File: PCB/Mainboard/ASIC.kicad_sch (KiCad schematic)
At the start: 0 parts

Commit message: Add files via upload
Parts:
- added U21: Bowman, symbol PC110:Bowman
- added U35: Pluto, symbol PC110:Pluto

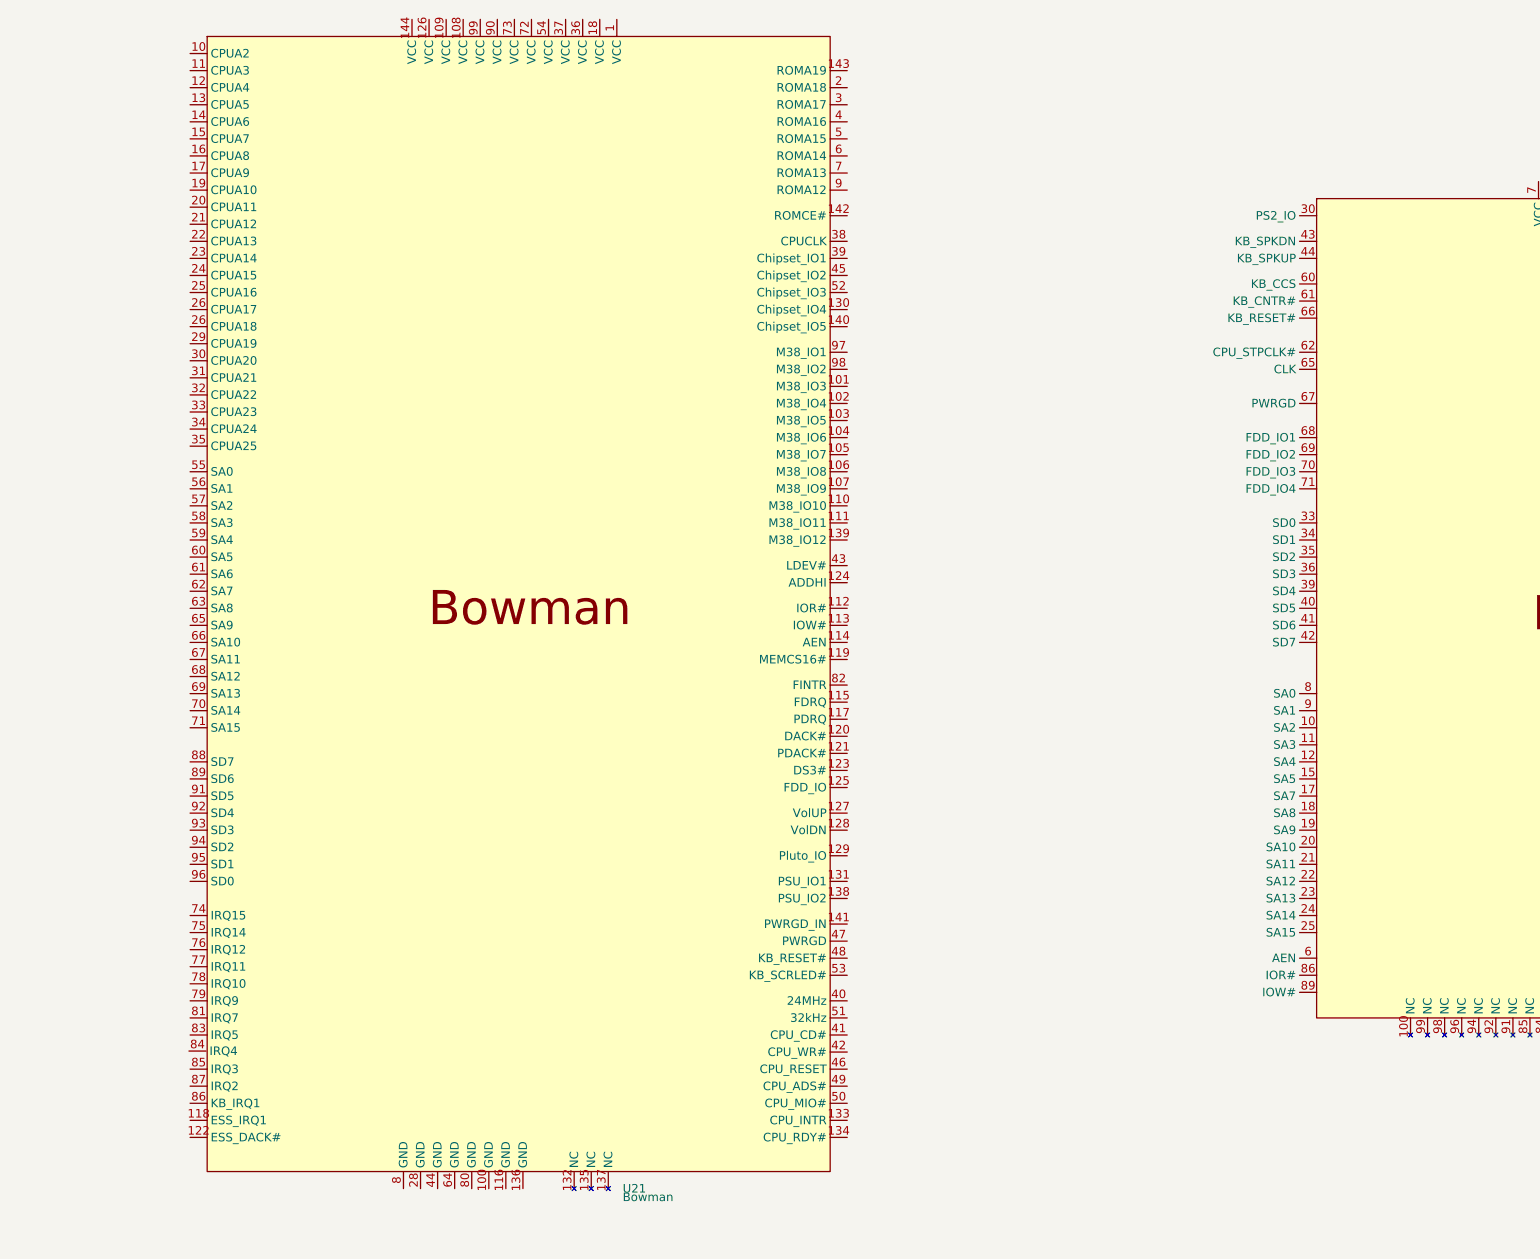
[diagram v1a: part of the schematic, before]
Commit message: Add files via upload
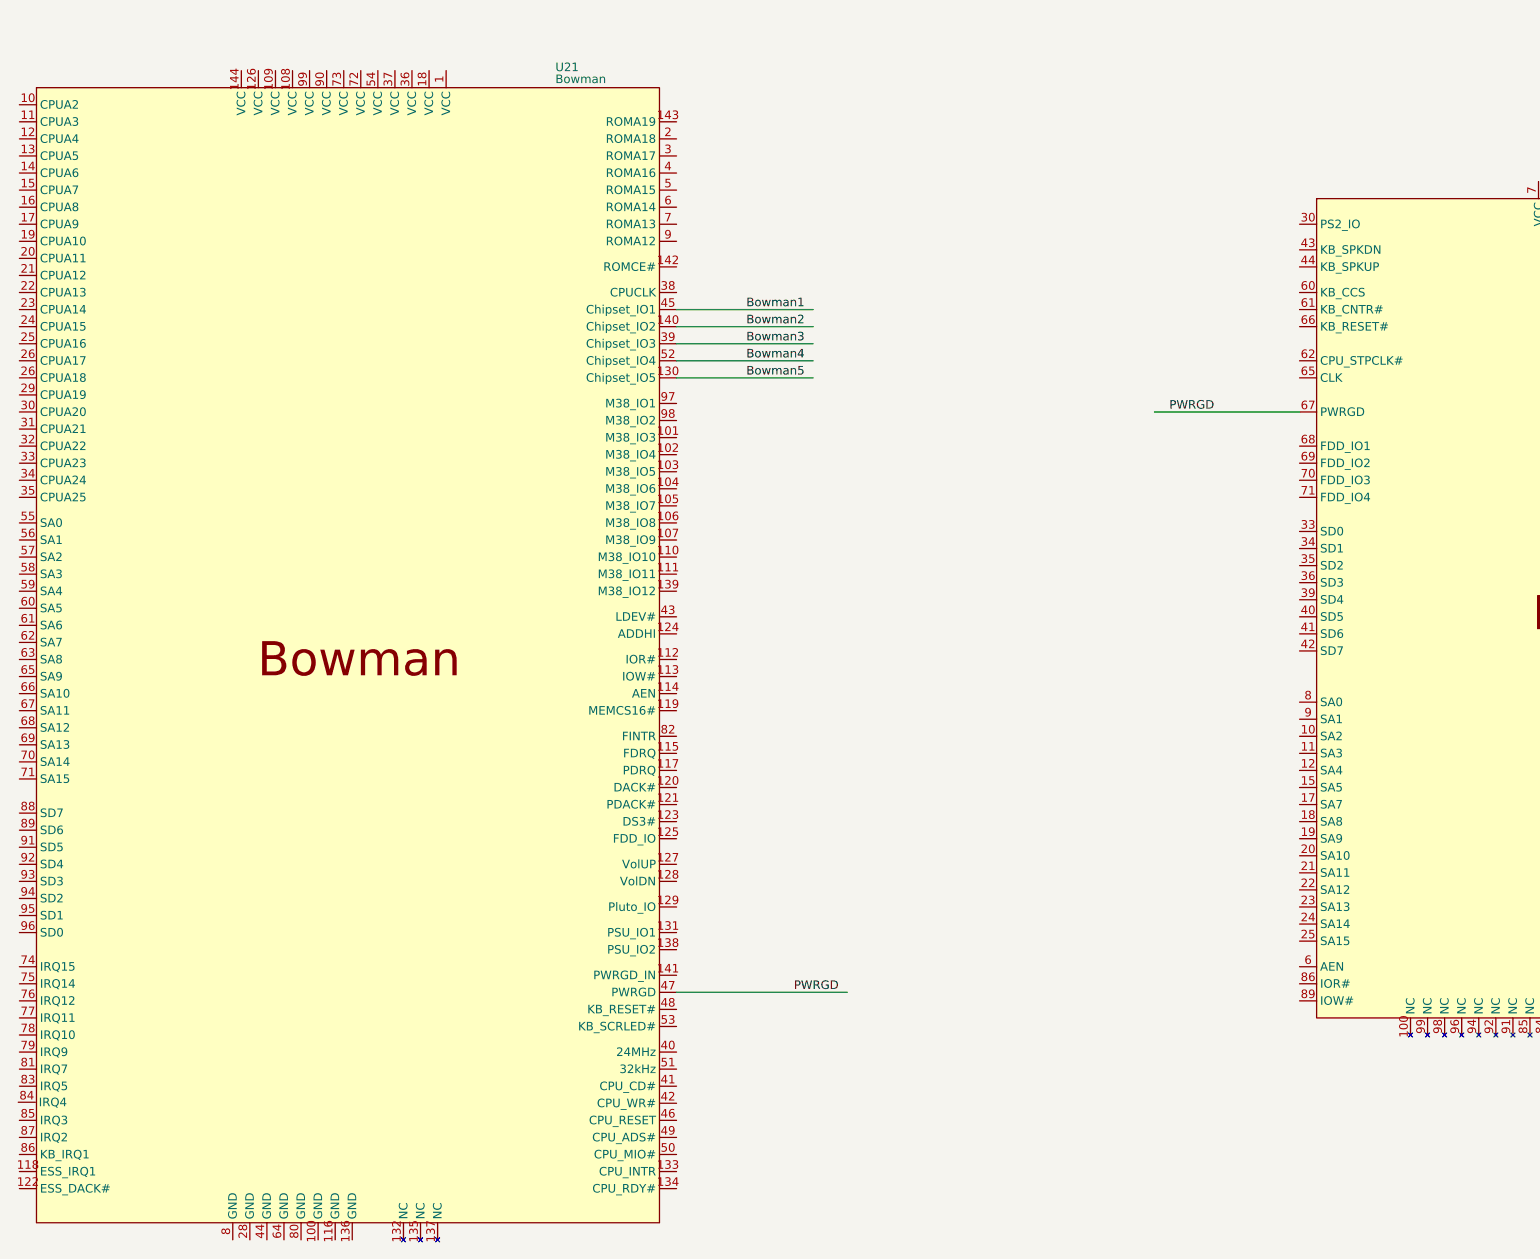
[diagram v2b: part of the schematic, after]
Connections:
- net PWRGD: now reaches U35.67 (PWRGD)
- net PWRGD: now also U21.47 (PWRGD)
- net Bowman5: now reaches U21.130 (Chipset_IO5)
- net Bowman2: now reaches U21.140 (Chipset_IO2)
- net Bowman3: now reaches U21.39 (Chipset_IO3)
- net Bowman1: now reaches U21.45 (Chipset_IO1)
- net Bowman4: now reaches U21.52 (Chipset_IO4)
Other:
- moved on the sheet: U21, U35
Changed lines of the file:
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@@
 		(title "PC110")
+	)
+	(wire
+		(pts
+			(xy 177.8 194.31) (xy 203.2 194.31)
+		)
+		(stroke
+			(width 0)
+			(type default)
+		)
+	)
+	(wire
+		(pts
+			(xy 248.92 107.95) (xy 270.51 107.95)
+		)
+		(stroke
+			(width 0)
+			(type default)
+		)
+	)
+	(wire
+		(pts
+			(xy 177.8 102.87) (xy 198.12 102.87)
+		)
+		(stroke
+			(width 0)
+			(type default)
+		)
+	)
+	(wire
+		(pts
+			(xy 177.8 95.25) (xy 198.12 95.25)
+		)
+		(stroke
+			(width 0)
+			(type default)
+		)
+	)
+	(wire
+		(pts
+			(xy 177.8 92.71) (xy 198.12 92.71)
+		)
+		(stroke
+			(width 0)
+			(type default)
+		)
+	)
+	(wire
+		(pts
+			(xy 177.8 97.79) (xy 198.12 97.79)
+		)
+		(stroke
+			(width 0)
+			(type default)
+		)
+	)
+	(wire
+		(pts
+			(xy 177.8 100.33) (xy 198.12 100.33)
+		)
+		(stroke
+			(width 0)
+			(type default)
+		)
+	)
+	(label "PWRGD"
+		(at 257.81 107.95 180)
+		(effects
+			(font
+				(size 1.27 1.27)
+			)
+			(justify right bottom)
+		)
+	)
+	(label "Bowman5"
+		(at 196.85 102.87 180)
+		(effects
+			(font
+				(size 1.27 1.27)
+			)
+			(justify right bottom)
+		)
+	)
+	(label "Bowman3"
+		(at 196.85 97.79 180)
+		(effects
+			(font
+				(size 1.27 1.27)
+			)
+			(justify right bottom)
+		)
+	)
+	(label "Bowman4"
+		(at 196.85 100.33 180)
+		(effects
+			(font
+				(size 1.27 1.27)
+			)
+			(justify right bottom)
+		)
+	)
+	(label "Bowman2"
+		(at 196.85 95.25 180)
+		(effects
+			(font
+				(size 1.27 1.27)
+			)
+			(justify right bottom)
+		)
+	)
+	(label "Bowman1"
+		(at 196.85 92.71 180)
+		(effects
+			(font
+				(size 1.27 1.27)
+			)
+			(justify right bottom)
+		)
+	)
+	(label "PWRGD"
+		(at 201.93 194.31 180)
+		(effects
+			(font
+				(size 1.27 1.27)
+			)
+			(justify right bottom)
+		)
 	)
 	(symbol
@@
 	(symbol
 		(lib_id "PC110:Bowman")
-		(at 153.67 138.43 0)
+		(at 128.27 146.05 0)
 		(unit 1)
 		(exclude_from_sim no)
@@
 		(on_board yes)
 		(dnp no)
-		(fields_autoplaced yes)
 		(property "Reference" "U21"
-			(at 169.7833 223.52 0)
+			(at 159.766 56.642 0)
 			(effects
 				(font
@@
 		)
 		(property "Value" "Bowman"
-			(at 169.7833 224.79 0)
+			(at 159.766 58.42 0)
 			(effects
 				(font
@@
 		)
 		(property "Footprint" ""
-			(at 153.67 138.43 0)
+			(at 128.27 146.05 0)
 			(effects
 				(font
@@
 		)
 		(property "Datasheet" ""
-			(at 153.67 138.43 0)
+			(at 128.27 146.05 0)
 			(effects
 				(font
@@
 		)
 		(property "Description" ""
-			(at 153.67 138.43 0)
-			(effects
-				(font
+			(at 128.27 146.05 0)
+			(effects
+				(font

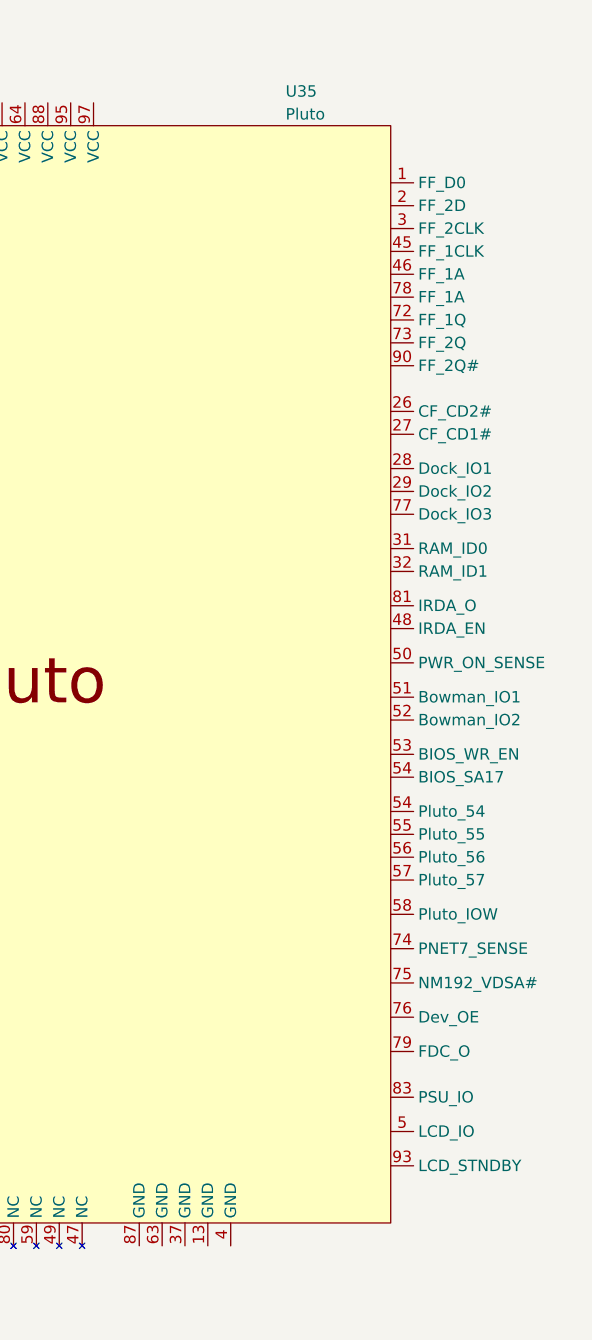
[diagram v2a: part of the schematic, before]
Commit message: Add files via upload
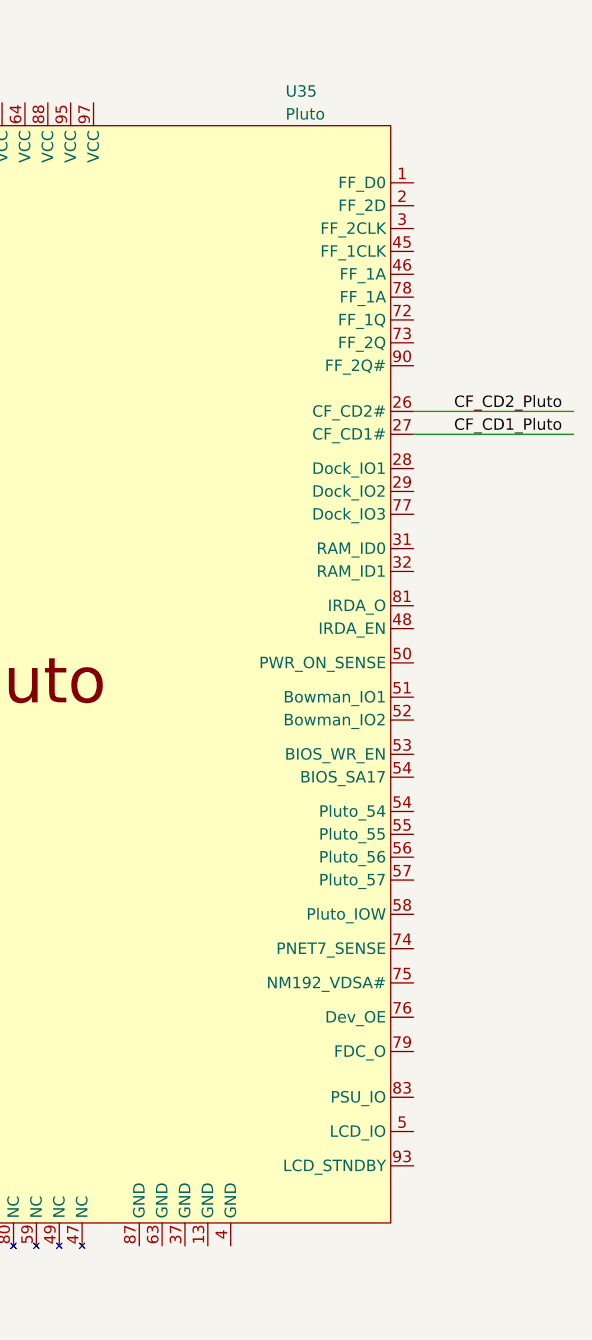
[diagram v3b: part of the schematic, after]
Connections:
- net CF_CD2_Pluto: now reaches U35.26 (CF_CD2#)
- net CF_CD1_Pluto: now reaches U35.27 (CF_CD1#)
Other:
- moved on the sheet: U35
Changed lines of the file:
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@@
+	(wire
+		(pts
+			(xy 356.87 110.49) (xy 374.65 110.49)
+		)
+		(stroke
+			(width 0)
+			(type default)
+		)
+	)
 	(wire
 		(pts
 			(xy 177.8 102.87) (xy 198.12 102.87)
+		)
+		(stroke
+			(width 0)
+			(type default)
+		)
+	)
+	(wire
+		(pts
+			(xy 356.87 107.95) (xy 374.65 107.95)
 		)
 		(stroke
@@
 		)
 	)
+	(label "CF_CD1_Pluto"
+		(at 373.38 110.49 180)
+		(effects
+			(font
+				(size 1.27 1.27)
+			)
+			(justify right bottom)
+		)
+	)
 	(label "Bowman2"
 		(at 196.85 95.25 180)
@@
 		(effects
 			(font
+				(size 1.27 1.27)
+			)
+			(justify right bottom)
+		)
+	)
+	(label "CF_CD2_Pluto"
+		(at 373.38 107.95 180)
+		(effects
+			(font

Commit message: Add files via upload
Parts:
- added C111, C125: 1nF, symbol Device:C
- added C117, C121, C127, C280: 100nF, symbol Device:C
- added C123, C128: 150nF, symbol Device:C
- added C130, C140, C277: 1uF, symbol Device:C
- added D33: N, symbol Device:D_Dual_CommonCathode_AKA
- added Q14, Q38: 8C, Package_TO_SOT_SMD:SOT-23, symbol Transistor_BJT:MMBTA44
- added R114, R393: 47k, symbol Device:R
- added R119, R182, R186, R215, R216: 470k, symbol Device:R
- added R257: 33, symbol Device:R
- added R382, R383: 50k, symbol Device:R
- added SW2: LidSwitch, symbol Switch:SW_SPST
- added U38: 7W14, symbol 74xGxx:74LVC3G14
- added U39: 7W00, symbol 74xGxx:74AHC2G00
- added U40: 74HC74, symbol 74xx:74HC74
- added U45: 74HC123, symbol 74xx:74HC123
- added U9: E4, symbol 74xGxx:74AHC1G32
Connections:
- net PWRGD: now also U38.3
- net GND: now reaches U35.13 (GND)
- net GND: now also U21.100 (GND), U21.116 (GND), U21.136 (GND), U21.28 (GND), U21.44 (GND), U21.64 (GND), U21.8 (GND), U21.80 (GND), U35.37 (GND), U35.4 (GND), U35.63 (GND), U35.87 (GND), C111.2, C117.2, C121.1, C123.1, C125.1, C127.1, C128.1, C277.2, C280.2, Q14.2 (E), Q38.2 (E), R186.1, R383.2, U38.4 (GND), U39.4 (GND), U40.7 (GND), U45.8 (GND), U45.9 (A), U9.3 (GND)
- net PNET1: now reaches U35.14 (VCC)
- net PNET1: now also U21.1 (VCC), U21.108 (VCC), U21.109 (VCC), U21.126 (VCC), U21.144 (VCC), U21.18 (VCC), U21.36 (VCC), U21.37 (VCC), U21.54 (VCC), U21.72 (VCC), U21.73 (VCC), U21.90 (VCC), U21.99 (VCC), U35.38 (VCC), U35.64 (VCC), U35.7 (VCC), U35.88 (VCC), U35.95 (VCC), U35.97 (VCC), C111.1, C117.1, C121.2, C123.2, C127.2, C128.2, C140.2, C280.1, R182.1, R215.1, R216.2, R393.1, SW2.1 (A), U38.8 (VCC), U39.8 (VCC), U40.13 (~{R}), U40.14 (VCC), U40.2 (D), U45.16 (VCC), U45.2 (B), U45.6 (Cext), U9.5 (VCC)
- net at U35.2 (FF_2D): now also R186.2, U40.12 (D)
- net U53_2CLK: now reaches U35.3 (FF_2CLK)
- net U53_2CLK: now also U40.11 (C)
- net at U35.45 (FF_1CLK): now also Q38.3 (C), R216.1, U38.1
- net FF_1A: now reaches U35.46 (FF_1A)
- net FF_1A: now also U35.78 (FF_1A), U45.1 (A)
- net CPU_STPCLK#: now reaches U35.62 (CPU_STPCLK#)
- net KB_RESET#: now reaches U35.66 (KB_RESET#)
- net KB_RESET#: now also U21.48 (KB_RESET#), U40.10 (~{S}), U40.4 (~{S}), U45.3 (Clr)
- net at U35.90 (FF_2Q#): now also U40.1 (~{R}), U45.12 (~{Q})
- net LCD_STNDBY#: now reaches U35.93 (LCD_STNDBY)
- net LCD_STNDBY#: now also R393.2
- net CPU_A2: now reaches U21.10 (CPUA2)
- net CPU_A3: now reaches U21.11 (CPUA3)
- net CPU_A4: now reaches U21.12 (CPUA4)
- net CPU_A5: now reaches U21.13 (CPUA5)
- net CPU_A6: now reaches U21.14 (CPUA6)
- net at U21.141 (PWRGD_IN): now also U9.4
- net CPU_A7: now reaches U21.15 (CPUA7)
- net CPU_A8: now reaches U21.16 (CPUA8)
- net CPU_A9: now reaches U21.17 (CPUA9)
- net CPU_A10: now reaches U21.19 (CPUA10)
- net CPU_A11: now reaches U21.20 (CPUA11)
- net CPU_A12: now reaches U21.21 (CPUA12)
- net CPU_A13: now reaches U21.22 (CPUA13)
- net CPU_A14: now reaches U21.23 (CPUA14)
- net CPU_A15: now reaches U21.24 (CPUA15)
- net CPU_A16: now reaches U21.25 (CPUA16)
- net CPU_A18: now reaches U21.26 (CPUA18)
- net CPU_A19: now reaches U21.29 (CPUA19)
- net CPU_A20: now reaches U21.30 (CPUA20)
- net CPU_A21: now reaches U21.31 (CPUA21)
- net CPU_A22: now reaches U21.32 (CPUA22)
- net CPU_A23: now reaches U21.33 (CPUA23)
- net CPU_A24: now reaches U21.34 (CPUA24)
- net CPU_A25: now reaches U21.35 (CPUA25)
- net at U21.38 (CPUCLK): now also R257.1
- net CPU_RESET: now reaches U21.46 (CPU_RESET)
- new net: R382.1, R383.1, SW2.2 (B)
- new net: C277.1, Q38.1 (B), R382.2
- new net: D33.1 (A), U45.5 (Q)
- new net: D33.2 (A), U45.13 (Q)
- new net: D33.3 (K), R114.2
- new net: C130.1, R182.2, U45.15 (RCext)
- new net: Q14.1 (B), R114.1
- new net: C130.2, U45.14 (Cext)
- new net: C140.1, R215.2, U45.7 (RCext)
- new net: C125.2, U39.1, U40.6 (~{Q})
- new net: U38.7, U39.2, U40.3 (C)
- new net: U39.7, U45.10 (B)
- new net: U38.5, U9.2
- new net: U40.8 (~{Q}), U45.11 (Clr)
- new net CPU_A17: U21.26 (CPUA18)
- new net CPU_SMIACT#: U9.1
- new net Chipset_CPU_CLK: R257.2
- new net RTCBAT: R119.1
- new net YMF_VSS_Res: Q14.3 (C), R119.2
- no-connect marks 0 -> 6
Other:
- moved on the sheet: U21, U35
